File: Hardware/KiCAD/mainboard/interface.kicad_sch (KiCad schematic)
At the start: 22 parts, among them J2 USB_C, J3 UART, J4 Conn_01x30, J5 STLink, Q1 BSS138, U5 USBLC6-2

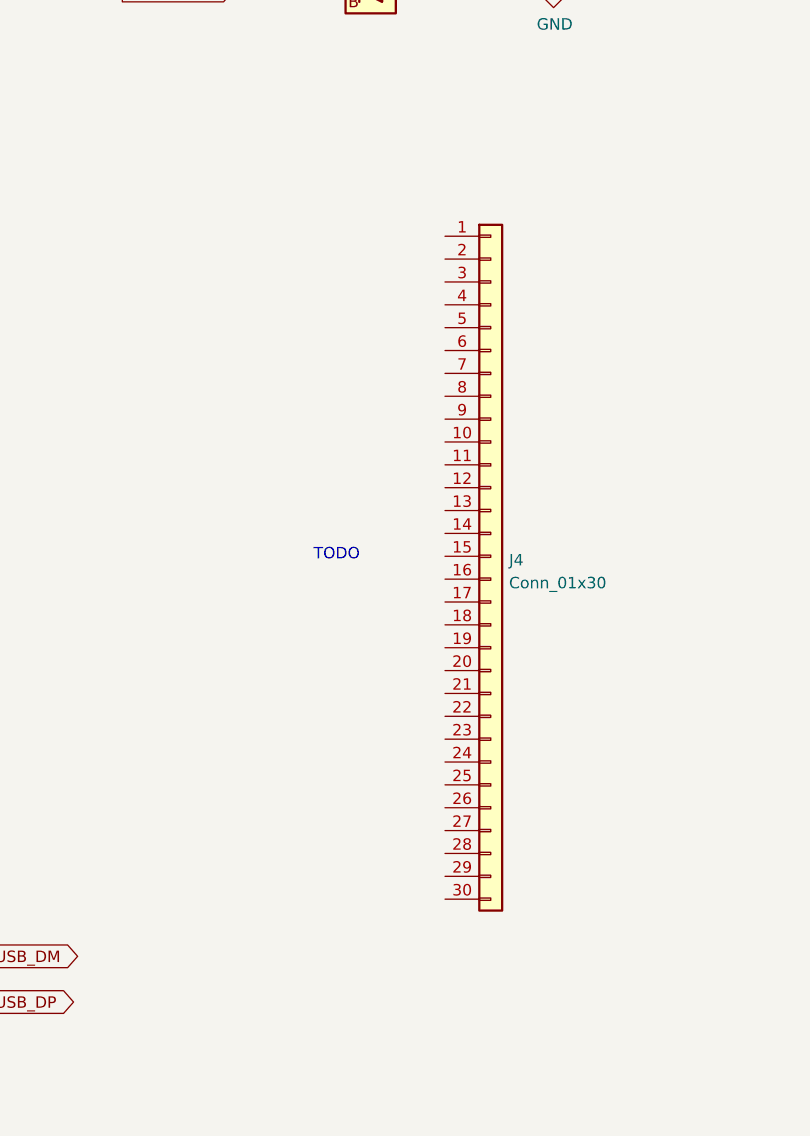
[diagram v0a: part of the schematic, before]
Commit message: Add files via upload
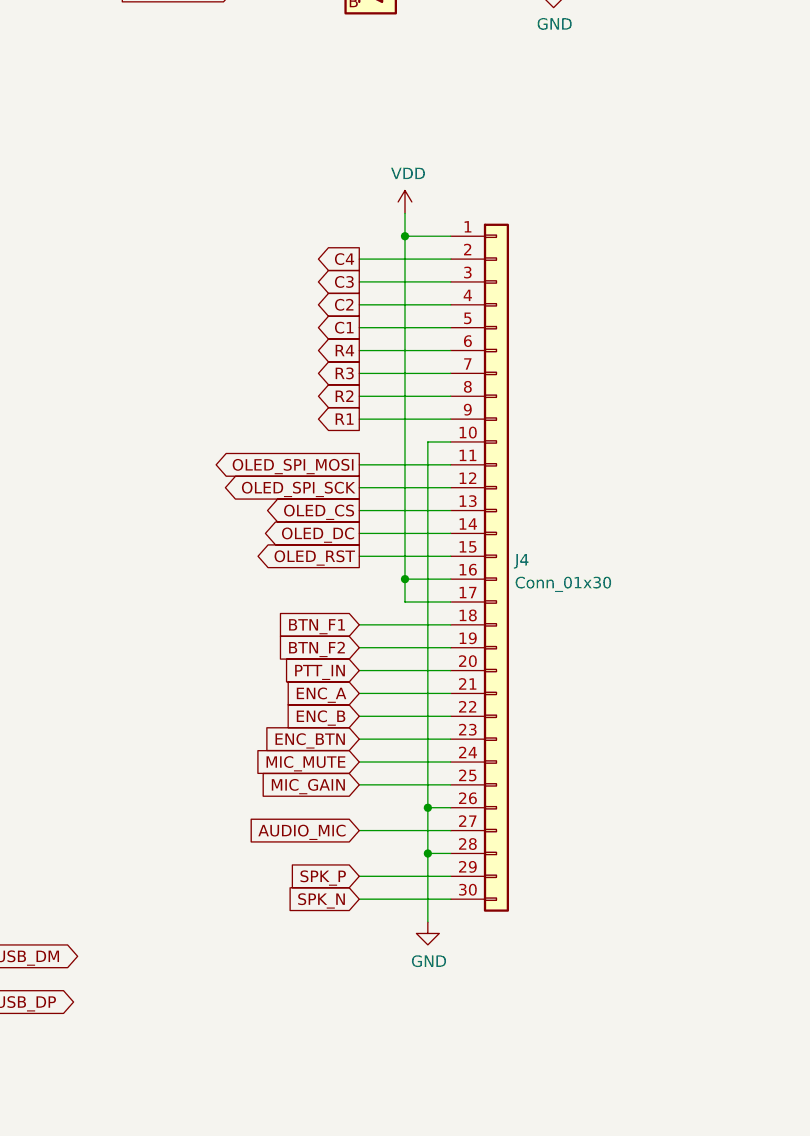
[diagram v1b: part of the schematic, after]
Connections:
- net BTN_F1: now also J4.18 (Pin_18)
- net GND: now also J4.10 (Pin_10), J4.26 (Pin_26), J4.28 (Pin_28)
- net VDD: now also J4.1 (Pin_1), J4.16 (Pin_16), J4.17 (Pin_17)
- net OLED_SPI_MOSI: now reaches J4.11 (Pin_11)
- net OLED_SPI_SCK: now reaches J4.12 (Pin_12)
- net OLED_CS: now reaches J4.13 (Pin_13)
- net OLED_DC: now reaches J4.14 (Pin_14)
- net OLED_RST: now reaches J4.15 (Pin_15)
- net BTN_F2: now reaches J4.19 (Pin_19)
- net C4: now reaches J4.2 (Pin_2)
- net PTT_IN: now reaches J4.20 (Pin_20)
- net ENC_A: now reaches J4.21 (Pin_21)
- net ENC_B: now reaches J4.22 (Pin_22)
- net ENC_BTN: now reaches J4.23 (Pin_23)
- net MIC_MUTE: now reaches J4.24 (Pin_24)
- net MIC_GAIN: now reaches J4.25 (Pin_25)
- net AUDIO_MIC: now reaches J4.27 (Pin_27)
- net SPK_P: now reaches J4.29 (Pin_29)
- net C3: now reaches J4.3 (Pin_3)
- net SPK_N: now reaches J4.30 (Pin_30)
- net C2: now reaches J4.4 (Pin_4)
- net C1: now reaches J4.5 (Pin_5)
- net R4: now reaches J4.6 (Pin_6)
- net R3: now reaches J4.7 (Pin_7)
- net R2: now reaches J4.8 (Pin_8)
- net R1: now reaches J4.9 (Pin_9)
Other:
- note removed: "TODO"
- moved on the sheet: J4
